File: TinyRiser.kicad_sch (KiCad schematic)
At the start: 25 parts, among them J2 Bus_PCI_Express_x16, J3 Bus_M.2_Socket_M, J4 fancontrol_header, M1 Fan_4pin

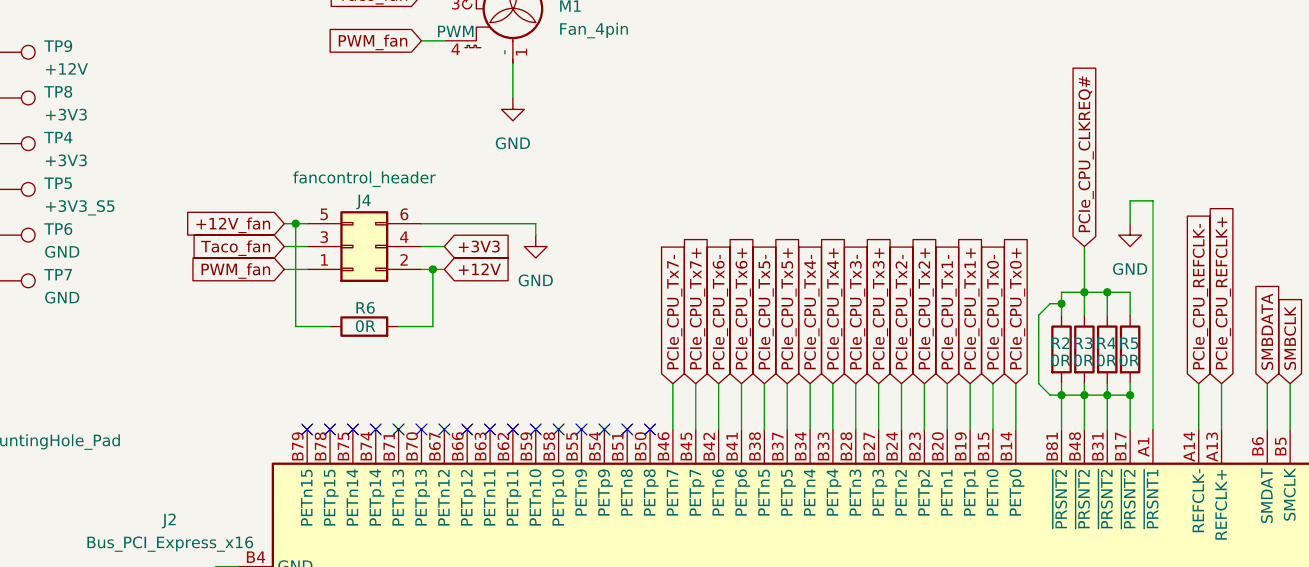
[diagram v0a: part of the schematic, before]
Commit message: Finished fan header implementation
Somehow it doesn't feel like it's done but it is???
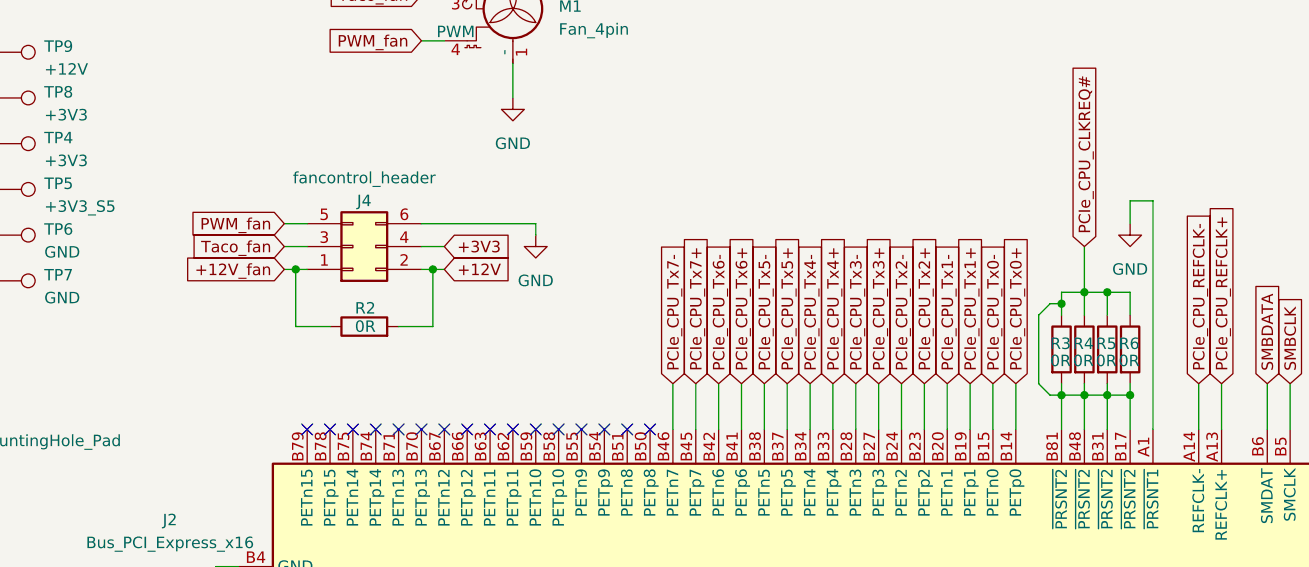
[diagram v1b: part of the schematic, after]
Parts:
- R2: renamed from R6; footprint Resistor_SMD:R_0603_1608Metric_Pad0.98x0.95mm_HandSolder -> Resistor_SMD:R_0805_2012Metric_Pad1.20x1.40mm_HandSolder
- renumbered R2 to R3, R3 to R4, R4 to R5, R5 to R6
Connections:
- net +12V_fan: now also J4.1 (Pin_1); no longer J4.5 (Pin_5)
- net PWM_fan: now also J4.5 (Pin_5); no longer J4.1 (Pin_1)
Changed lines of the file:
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@@
 	)
 	(junction
-		(at 203.2 52.07)
-		(diameter 0)
-		(color 0 0 0 0)
-	)
-	(junction
 		(at 130.81 224.79)
 		(diameter 0)
@@
 	)
 	(junction
+		(at 203.2 57.15)
+		(diameter 0)
+		(color 0 0 0 0)
+	)
+	(junction
 		(at 238.76 176.53)
 		(diameter 0)
@@
 	(wire
 		(pts
+			(xy 203.2 57.15) (xy 204.47 57.15)
+		)
+		(stroke
+			(width 0)
+			(type default)
+		)
+	)
+	(wire
+		(pts
 			(xy 213.36 223.52) (xy 213.36 228.6)
 		)
@@
 	(wire
 		(pts
-			(xy 203.2 52.07) (xy 204.47 52.07)
+			(xy 201.93 52.07) (xy 204.47 52.07)
 		)
 		(stroke
@@
 	(wire
 		(pts
-			(xy 201.93 52.07) (xy 203.2 52.07)
-		)
-		(stroke
-			(width 0)
-			(type default)
-		)
-	)
-	(wire
-		(pts
 			(xy 246.38 176.53) (xy 251.46 176.53)
 		)
@@
 	(wire
 		(pts
+			(xy 203.2 63.5) (xy 203.2 57.15)
+		)
+		(stroke
+			(width 0)
+			(type default)
+		)
+	)
+	(wire
+		(pts
 			(xy 107.95 102.87) (xy 113.03 102.87)
 		)
@@
 	(wire
 		(pts
-			(xy 201.93 57.15) (xy 204.47 57.15)
+			(xy 201.93 57.15) (xy 203.2 57.15)
 		)
 		(stroke
@@
 	(wire
 		(pts
-			(xy 203.2 63.5) (xy 203.2 52.07)
-		)
-		(stroke
-			(width 0)
-			(type default)
-		)
-	)
-	(wire
-		(pts
 			(xy 170.18 172.72) (xy 170.18 177.8)
 		)
@@
 	(global_label "+12V_fan"
 		(shape input)
-		(at 201.93 52.07 180)
+		(at 201.93 57.15 180)
 		(fields_autoplaced yes)
 		(effects
@@
 		)
 		(property "Intersheetrefs" "${INTERSHEET_REFS}"
-			(at 189.8735 52.07 0)
+			(at 189.8735 57.15 0)
 			(effects
 				(font
@@
 	(global_label "PWM_fan"
 		(shape input)
-		(at 201.93 57.15 180)
+		(at 201.93 52.07 180)
 		(fields_autoplaced yes)
 		(effects
@@
 		)
 		(property "Intersheetrefs" "${INTERSHEET_REFS}"
-			(at 190.7807 57.15 0)
+			(at 190.7807 52.07 0)
 			(effects
 				(font
@@
 		(on_board yes)
 		(dnp no)
-		(property "Reference" "R4"
+		(property "Reference" "R5"
 			(at 292.1 65.405 0)
 			(effects
@@
 			(project "TinyRiser"
 				(path "/881240ea-c4b5-4af2-848a-893b6d69814c"
-					(reference "R4")
+					(reference "R5")
 					(unit 1)
 				)
@@
 		(on_board yes)
 		(dnp no)
-		(property "Reference" "R2"
+		(property "Reference" "R3"
 			(at 287.02 65.405 0)
 			(effects
@@
 			(project "TinyRiser"
 				(path "/881240ea-c4b5-4af2-848a-893b6d69814c"
-					(reference "R2")
+					(reference "R3")
 					(unit 1)
 				)
@@
 		(on_board yes)
 		(dnp no)
-		(property "Reference" "R6"
+		(property "Reference" "R2"
 			(at 212.09 61.468 90)
 			(effects
@@
 			)
 		)
-		(property "Footprint" "Resistor_SMD:R_0603_1608Metric_Pad0.98x0.95mm_HandSolder"
+		(property "Footprint" "Resistor_SMD:R_0805_2012Metric_Pad1.20x1.40mm_HandSolder"
 			(at 210.82 65.278 90)
 			(effects
@@
 			(project "TinyRiser"
 				(path "/881240ea-c4b5-4af2-848a-893b6d69814c"
-					(reference "R6")
+					(reference "R2")
 					(unit 1)
 				)
@@
 		(on_board yes)
 		(dnp no)
-		(property "Reference" "R3"
+		(property "Reference" "R4"
 			(at 289.56 65.405 0)
 			(effects
@@
 			(project "TinyRiser"
 				(path "/881240ea-c4b5-4af2-848a-893b6d69814c"
-					(reference "R3")
+					(reference "R4")
 					(unit 1)
 				)
@@
 		(on_board yes)
 		(dnp no)
-		(property "Reference" "R5"
+		(property "Reference" "R6"
 			(at 294.64 65.405 0)
 			(effects
@@
 			(project "TinyRiser"
 				(path "/881240ea-c4b5-4af2-848a-893b6d69814c"
-					(reference "R5")
+					(reference "R6")
 					(unit 1)
 				)
